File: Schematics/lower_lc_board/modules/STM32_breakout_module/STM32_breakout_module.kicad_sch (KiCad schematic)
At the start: 54 parts, among them J2 SWD_CONN, J3 USB_C_CONN, Q4 2N7002, SW1 SW_STM_RESET, SW2 SW_STM_BOOT_MODE, U5 STM32F103CBT6, U6 W25Q128JVS, U7 ISO1044BDR, U8 CP2102N-Axx-xQFN28, Y1 X322516MMB4SI

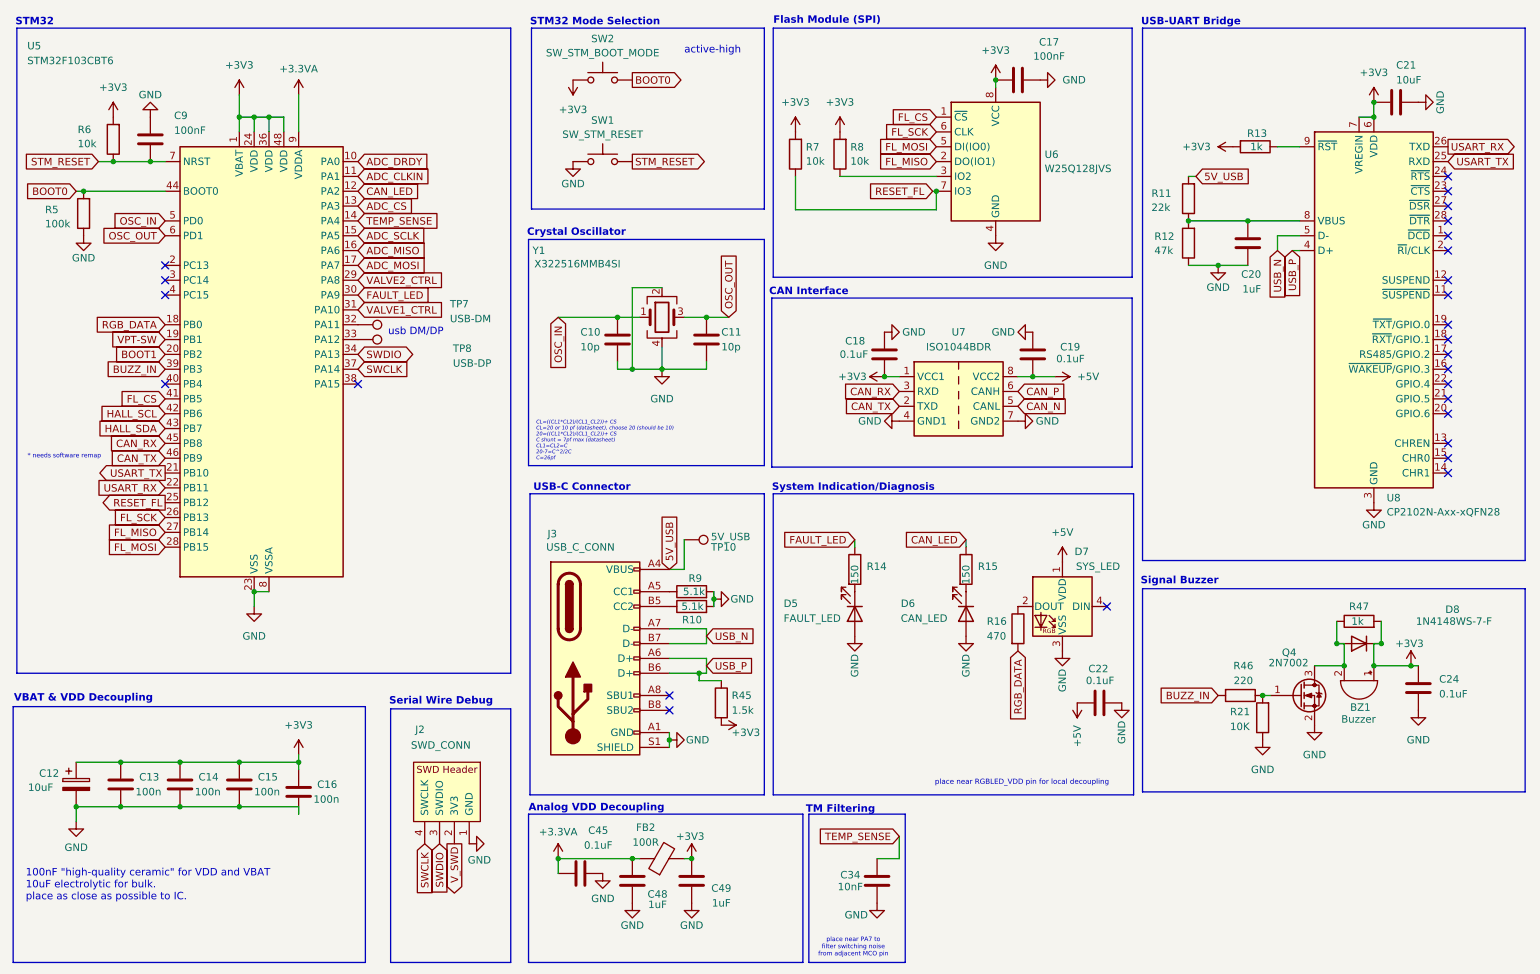
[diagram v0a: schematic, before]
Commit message: routing work
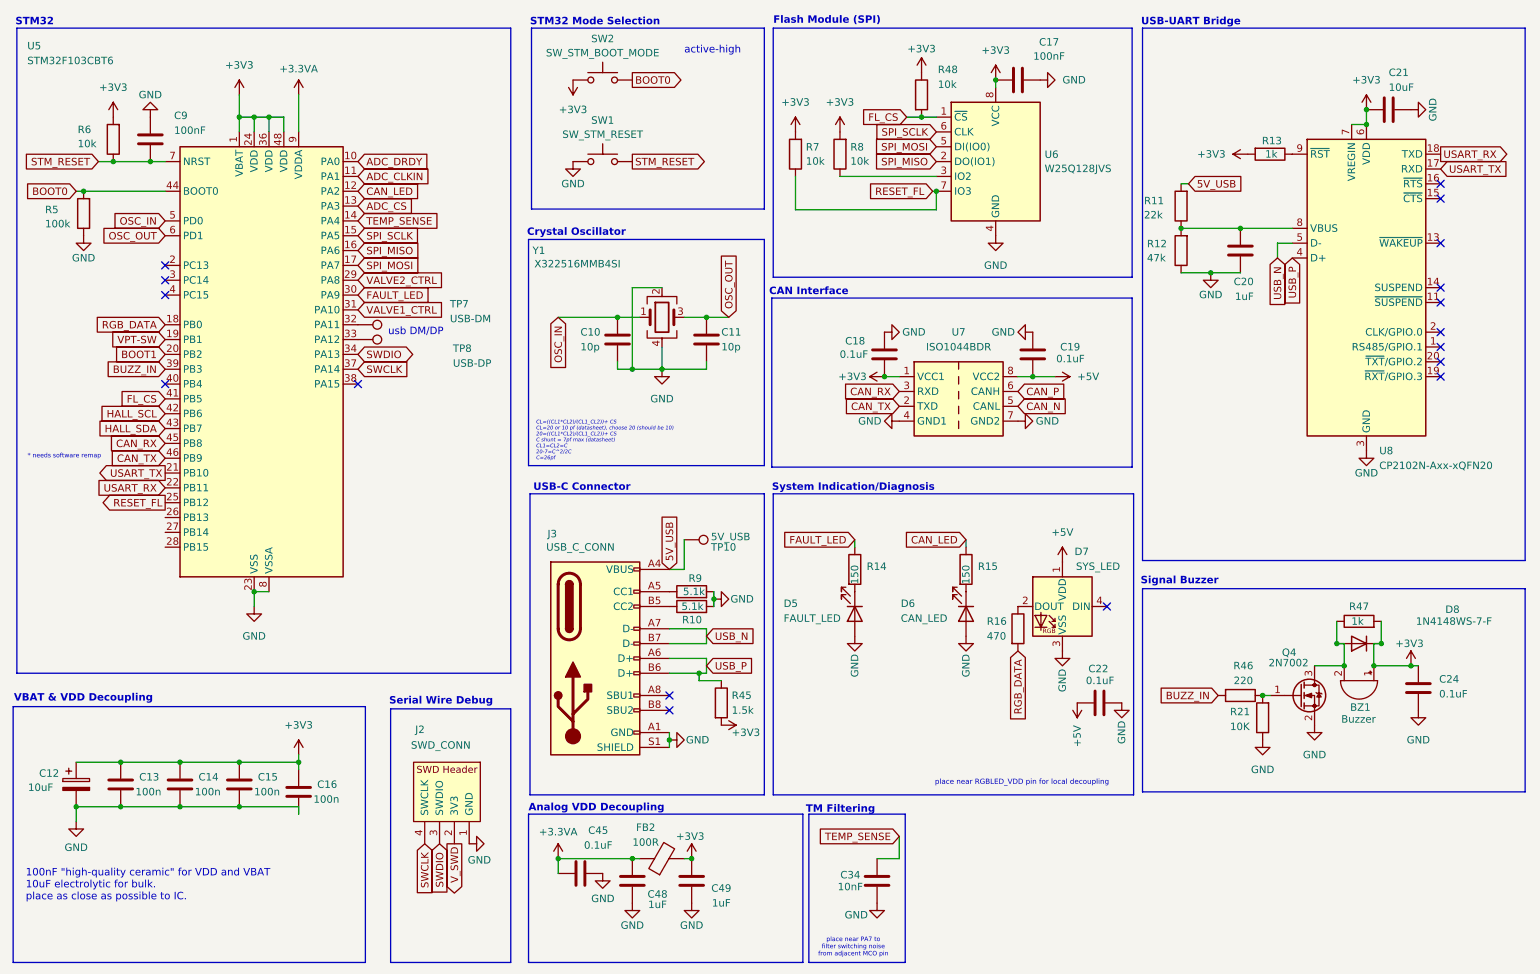
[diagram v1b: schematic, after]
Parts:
- removed U8: CP2102N-Axx-xQFN28, Package_DFN_QFN:QFN-28-1EP_5x5mm_P0.5mm_EP3.35x3.35mm, symbol Interface_USB:CP2102N-Axx-xQFN28
- added R48: 10k, Resistor_SMD:R_0402_1005Metric, symbol Device:R
- added U8: CP2102N-Axx-xQFN20, CP2102N_A02_GQFN20:QFN20_CP2102N_SIL, symbol Interface_USB:CP2102N-Axx-xQFN20
- C45: footprint Capacitor_SMD:C_0805_2012Metric -> Capacitor_SMD:C_0603_1608Metric; JLCPCB (none) -> C14663
- C48, C49: footprint Capacitor_SMD:C_0805_2012Metric -> Capacitor_SMD:C_0603_1608Metric; JLCPCB C28323 -> C15849
- R10, R9: footprint Resistor_SMD:R_0603_1608Metric -> Resistor_SMD:R_0402_1005Metric; JLCPCB (none) -> C25905
- R11: footprint Resistor_SMD:R_0603_1608Metric -> Resistor_SMD:R_0402_1005Metric; JLCPCB C31850 -> C25768
- R12: footprint Resistor_SMD:R_0603_1608Metric -> Resistor_SMD:R_0402_1005Metric; JLCPCB C25819 -> C25792
- R13: footprint Resistor_SMD:R_0603_1608Metric -> Capacitor_SMD:C_0402_1005Metric; JLCPCB C21190 -> C11702
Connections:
- net +3V3: now also R48.1, U8.6 (VDD), U8.7 (VREGIN)
- net FL_CS: now also R48.2
- net GND: now also U8.12 (GND), U8.21 (GND), U8.3 (GND)
- net USART_RX: now also U8.18 (TXD)
- net USART_TX: now also U8.17 (RXD)
- net USB_N: now also U8.5 (D-)
- net USB_P: now also U8.4 (D+)
- net at C20.2, R11.1, R12.2: now also U8.8 (VBUS)
- net at R13.1: now also U8.9 (~{RST})
- net ADC_MISO renamed SPI_MISO
- net SPI_MISO: now also U6.2 (DO(IO1))
- net ADC_MOSI renamed SPI_MOSI
- net SPI_MOSI: now also U6.5 (DI(IO0))
- net ADC_SCLK renamed SPI_SCLK
- net SPI_SCLK: now also U6.6 (CLK)
- net FL_MISO: no longer names the net of U5.27 (PB14)
- net FL_MISO: no longer U6.2 (DO(IO1))
- net FL_MOSI: no longer names the net of U5.28 (PB15)
- net FL_MOSI: no longer U6.5 (DI(IO0))
- net FL_SCK: no longer names the net of U5.26 (PB13)
- net FL_SCK: no longer U6.6 (CLK)
- no-connect marks 26 -> 17

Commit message: routing work
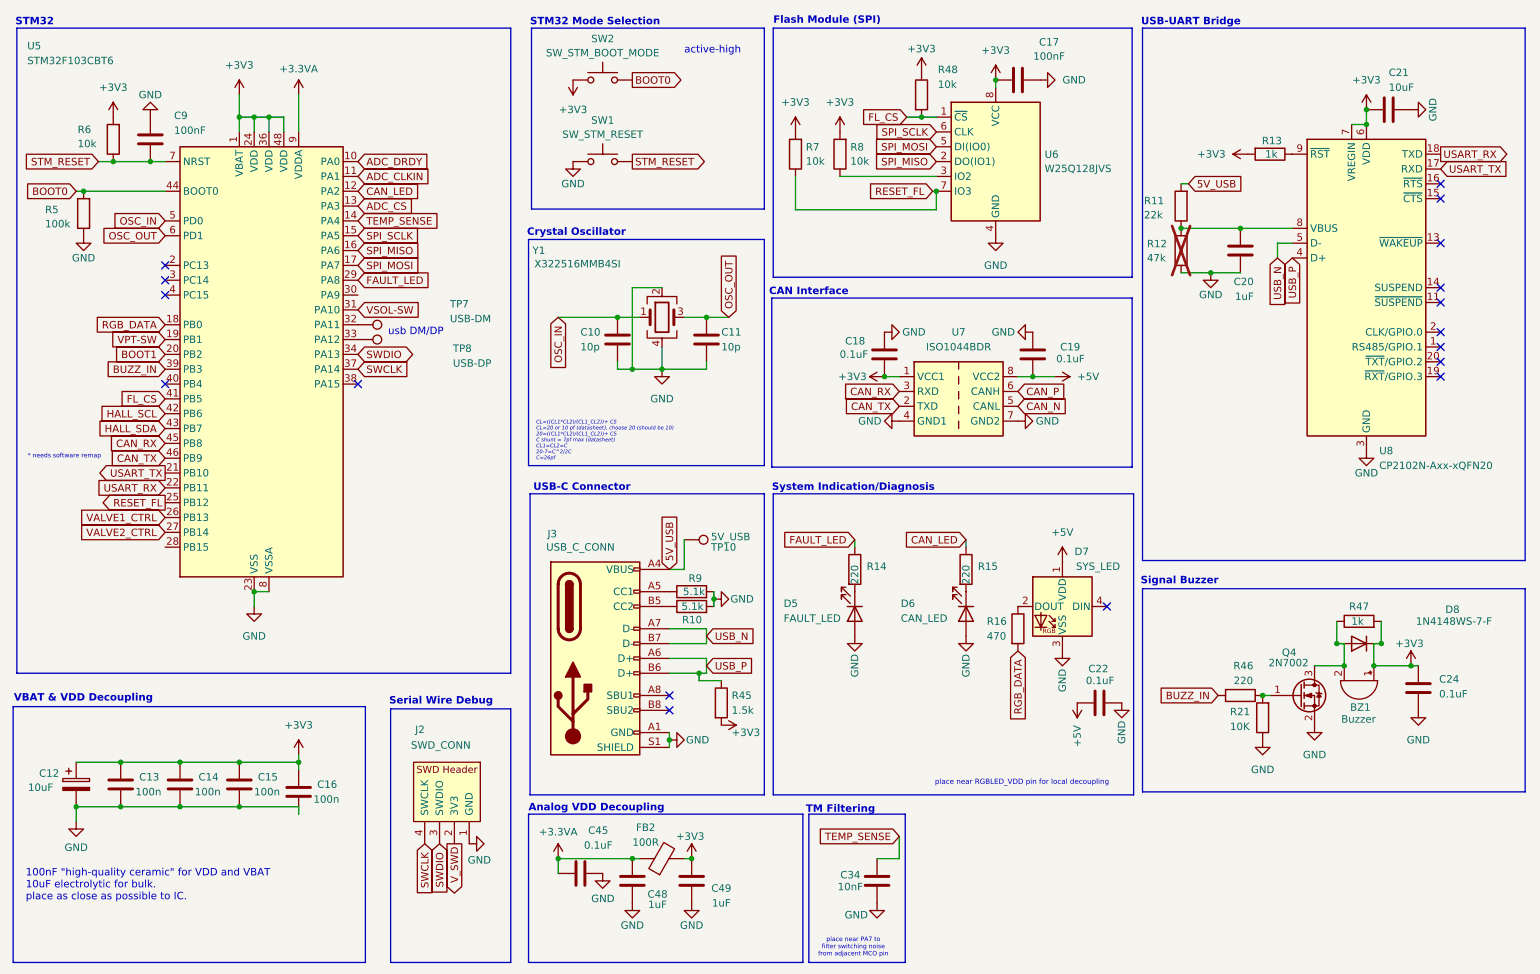
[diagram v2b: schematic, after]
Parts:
- R12: now not fitted
- R14, R15: value 150 -> 220; footprint Resistor_SMD:R_0603_1608Metric -> Resistor_SMD:R_0402_1005Metric; JLCPCB (none) -> C25104
- R46: JLCPCB (none) -> C25104
- TP7, TP8: footprint TestPoint:TestPoint_Pad_1.0x1.0mm -> TestPoint:TestPoint_Pad_D1.0mm
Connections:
- net FAULT_LED: now also U5.29 (PA8); no longer U5.30 (PA9)
- net VALVE1_CTRL: now also U5.26 (PB13); no longer U5.31 (PA10)
- net VALVE2_CTRL: now also U5.27 (PB14); no longer U5.29 (PA8)
- new net VSOL-SW: U5.31 (PA10)
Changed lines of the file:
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@@
 		)
 	)
+	(global_label "FAULT_LED"
+		(shape input)
+		(at 74.93 68.58 0)
+		(fields_autoplaced yes)
+		(effects
+			(font
+				(size 1.27 1.27)
+			)
+			(justify left)
+		)
+		(property "Intersheetrefs" "${INTERSHEET_REFS}"
+			(at 87.8333 68.58 0)
+			(effects
+				(font
+					(size 1.27 1.27)
+				)
+				(justify left)
+				(hide yes)
+			)
+		)
+	)
 	(global_label "SWCLK"
 		(shape input)
@@
 		)
 	)
+	(global_label "VSOL-SW"
+		(shape input)
+		(at 74.93 73.66 0)
+		(fields_autoplaced yes)
+		(effects
+			(font
+				(size 1.27 1.27)
+			)
+			(justify left)
+		)
+		(property "Intersheetrefs" "${INTERSHEET_REFS}"
+			(at 86.8052 73.66 0)
+			(effects
+				(font
+					(size 1.27 1.27)
+				)
+				(justify left)
+				(hide yes)
+			)
+		)
+	)
 	(global_label "BOOT0"
 		(shape output)
@@
 		)
 	)
-	(global_label "VALVE1_CTRL"
-		(shape input)
-		(at 74.93 73.66 0)
-		(fields_autoplaced yes)
-		(effects
-			(font
-				(size 1.27 1.27)
-			)
-			(justify left)
-		)
-		(property "Intersheetrefs" "${INTERSHEET_REFS}"
-			(at 90.0709 73.66 0)
-			(effects
-				(font
-					(size 1.27 1.27)
-				)
-				(justify left)
-				(hide yes)
-			)
-		)
-	)
 	(global_label "BUZZ_IN"
 		(shape input)
@@
 		)
 	)
-	(global_label "FAULT_LED"
+	(global_label "VALVE2_CTRL"
 		(shape input)
-		(at 74.93 71.12 0)
+		(at 41.91 111.76 180)
 		(fields_autoplaced yes)
 		(effects
@@
 				(size 1.27 1.27)
 			)
-			(justify left)
+			(justify right)
 		)
 		(property "Intersheetrefs" "${INTERSHEET_REFS}"
-			(at 87.8333 71.12 0)
+			(at 26.7691 111.76 0)
 			(effects
 				(font
 					(size 1.27 1.27)
 				)
-				(justify left)
+				(justify right)
 				(hide yes)
 			)
@@
 		)
 	)
-	(global_label "VALVE2_CTRL"
-		(shape input)
-		(at 74.93 68.58 0)
-		(fields_autoplaced yes)
-		(effects
-			(font
-				(size 1.27 1.27)
-			)
-			(justify left)
-		)
-		(property "Intersheetrefs" "${INTERSHEET_REFS}"
-			(at 90.0709 68.58 0)
-			(effects
-				(font
-					(size 1.27 1.27)
-				)
-				(justify left)
-				(hide yes)
-			)
-		)
-	)
 	(global_label "RESET_FL"
 		(shape output)
@@
 		)
 	)
+	(global_label "VALVE1_CTRL"
+		(shape input)
+		(at 41.91 109.22 180)
+		(fields_autoplaced yes)
+		(effects
+			(font
+				(size 1.27 1.27)
+			)
+			(justify right)
+		)
+		(property "Intersheetrefs" "${INTERSHEET_REFS}"
+			(at 26.7691 109.22 0)
+			(effects
+				(font
+					(size 1.27 1.27)
+				)
+				(justify right)
+				(hide yes)
+			)
+		)
+	)
 	(symbol
 		(lib_id "Device:C_Polarized")
@@
 			)
 		)
+		(property "JLCPCB" "C25104"
+			(at 226.06 139.7 0)
+			(effects
+				(font
+					(size 1.27 1.27)
+				)
+				(hide yes)
+			)
+		)
 		(pin "2"
 		)
@@
 			)
 		)
-		(property "Value" "150"
+		(property "Value" "220"
 			(at 179.07 120.65 90)
 			(effects
@@
 			)
 		)
-		(property "Footprint" "Resistor_SMD:R_0603_1608Metric"
+		(property "Footprint" "Resistor_SMD:R_0402_1005Metric"
 			(at 177.292 118.11 90)
 			(effects
@@
 			)
 		)
+		(property "JLCPCB" "C25104"
+			(at 179.07 118.11 0)
+			(effects
+				(font
+					(size 1.27 1.27)
+				)
+				(hide yes)
+			)
+		)
 		(pin "2"
 		)
@@
 			)
 		)
-		(property "Footprint" "TestPoint:TestPoint_Pad_1.0x1.0mm"
+		(property "Footprint" "TestPoint:TestPoint_Pad_D1.0mm"
 			(at 74.93 81.28 0)
 			(effects
@@
 		(in_bom yes)
 		(on_board yes)
-		(dnp no)
+		(dnp yes)
 		(property "Reference" "R12"
 			(at 210.058 62.3458 0)
@@
 			)
 		)
-		(property "Value" "150"
+		(property "Value" "220"
 			(at 160.02 120.65 90)
 			(effects
@@
 			)
 		)
-		(property "Footprint" "Resistor_SMD:R_0603_1608Metric"
+		(property "Footprint" "Resistor_SMD:R_0402_1005Metric"
 			(at 158.242 118.11 90)
 			(effects
@@
 			)
 		)
+		(property "JLCPCB" "C25104"
+			(at 160.02 118.11 0)
+			(effects
+				(font
+					(size 1.27 1.27)
+				)
+				(hide yes)
+			)
+		)
 		(pin "2"
 		)
@@
 			)
 		)
-		(property "Footprint" "TestPoint:TestPoint_Pad_1.0x1.0mm"
+		(property "Footprint" "TestPoint:TestPoint_Pad_D1.0mm"
 			(at 74.93 83.82 0)
 			(effects

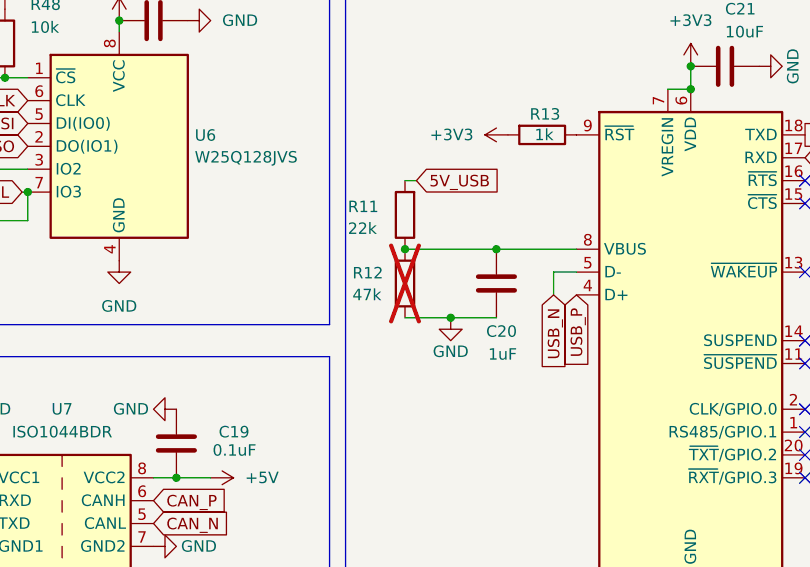
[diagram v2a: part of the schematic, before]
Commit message: routing work
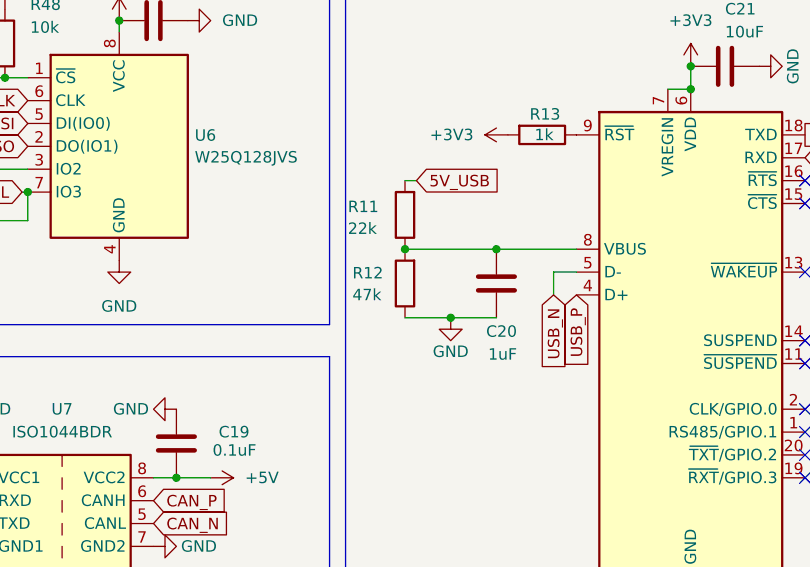
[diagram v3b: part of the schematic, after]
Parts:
- R12: now fitted
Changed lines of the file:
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@@
 		(in_bom yes)
 		(on_board yes)
-		(dnp yes)
+		(dnp no)
 		(property "Reference" "R12"
 			(at 210.058 62.3458 0)
